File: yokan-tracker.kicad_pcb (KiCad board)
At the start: 2 copper layers, 50 x 25 mm, 3 parts, among them U1 XIAO_ESP32_C6, U2 LSM6DSV_Module

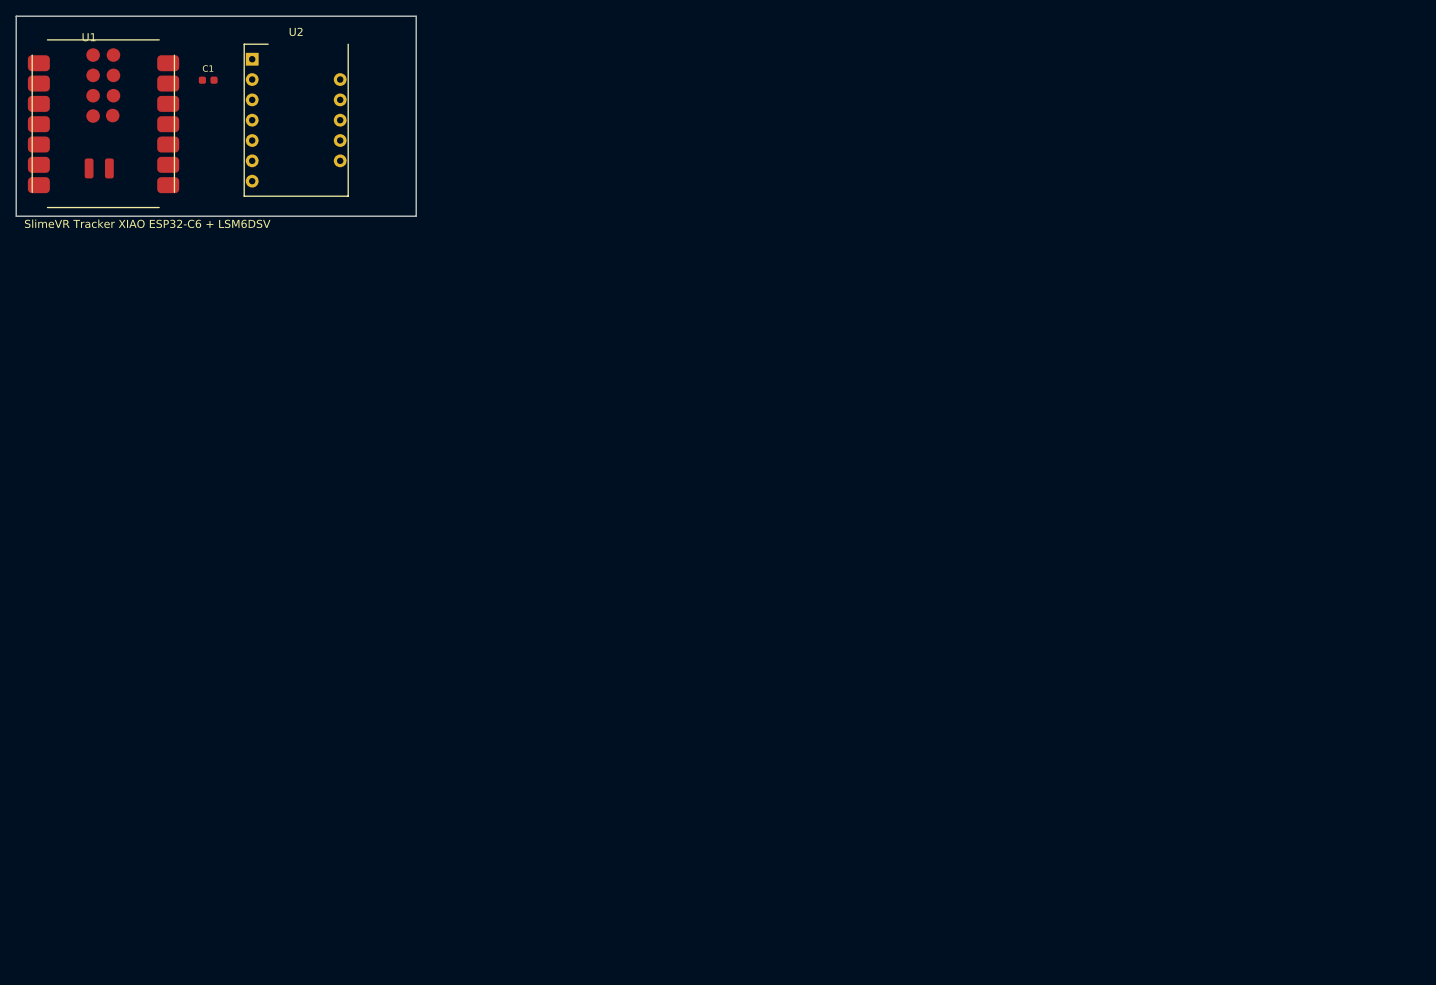
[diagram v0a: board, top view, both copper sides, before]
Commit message: バージョン対応
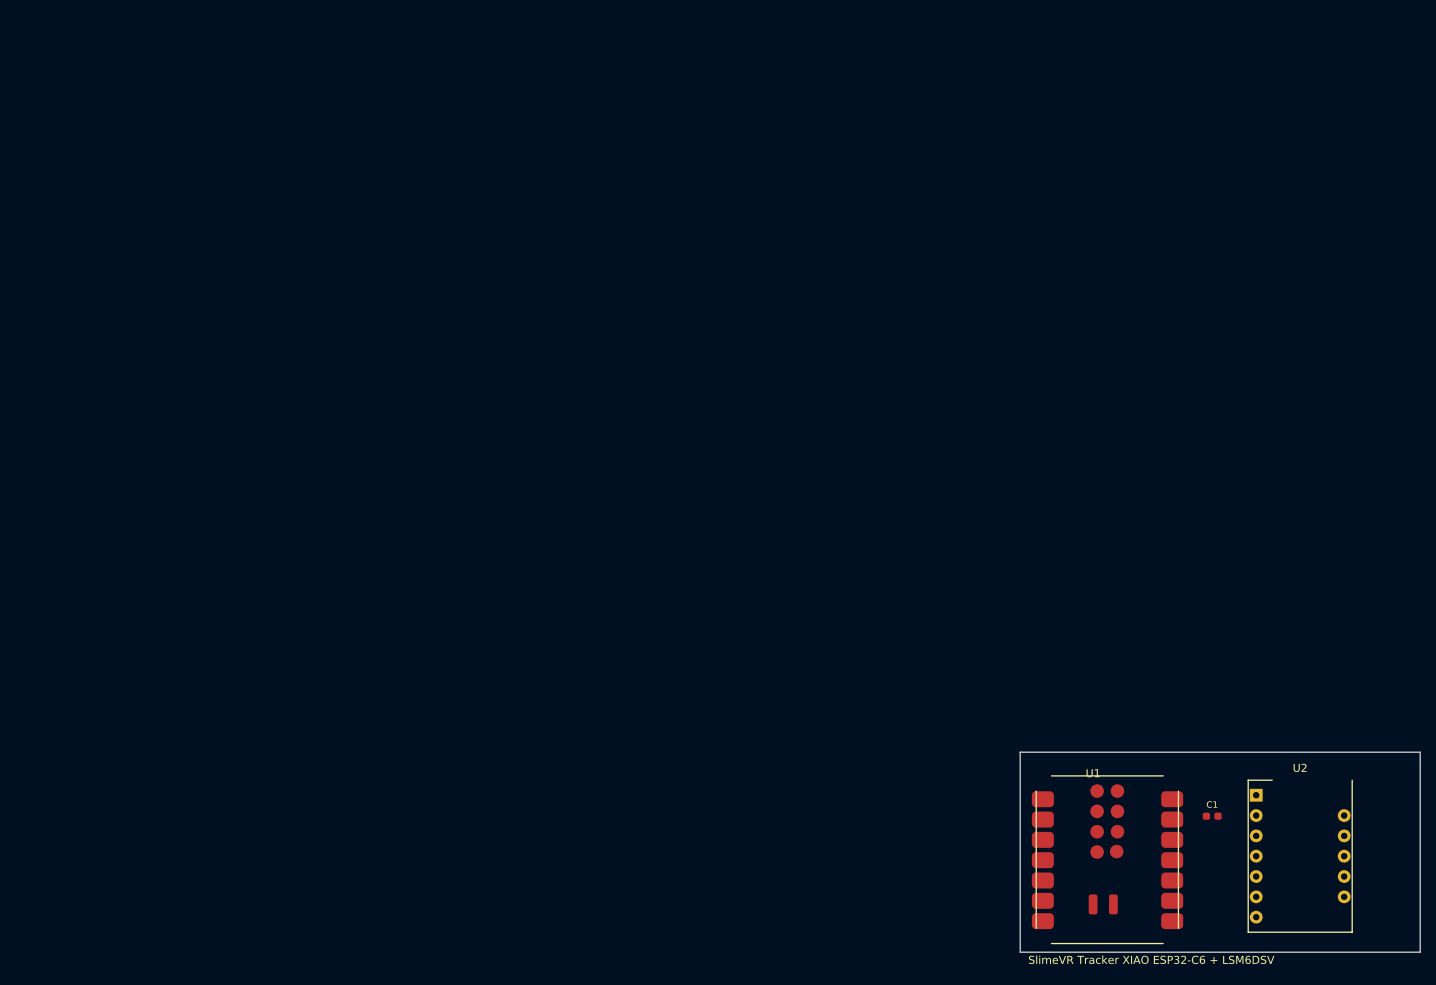
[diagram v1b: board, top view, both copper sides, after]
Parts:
- moved C1 155.6 mm to (149.5, 100.0)
- moved U1 155.6 mm to (127.5, 116.0)
- moved U2 155.6 mm to (160.5, 105.0)
